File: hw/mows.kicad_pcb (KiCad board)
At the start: 2 copper layers, 47 x 50.8 mm, 18 parts, among them J1 ICSP, J2 STX882, J3 DHT22, J4 WSPD, J5 WDIR, J6 RAIN, U1 MCP1700, U2 ATTINY85-20PU

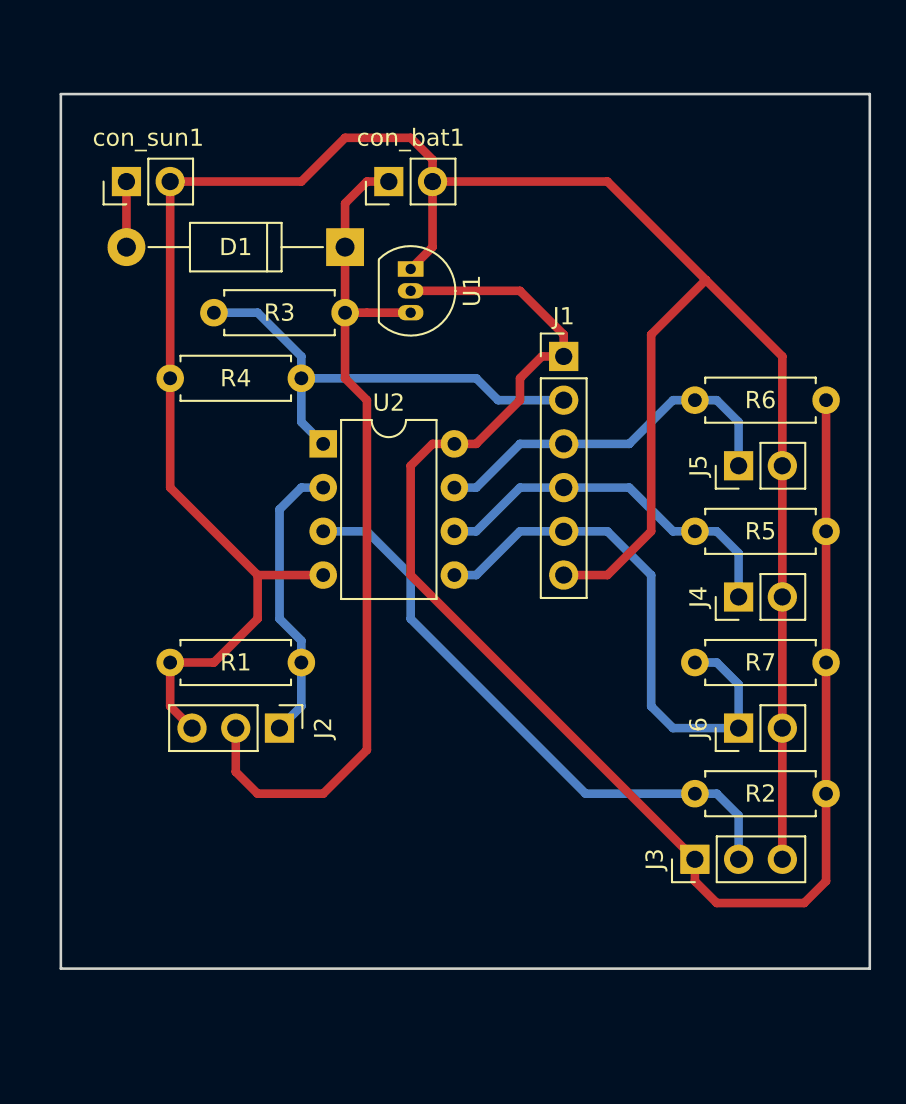
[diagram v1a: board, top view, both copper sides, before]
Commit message: Nova placa
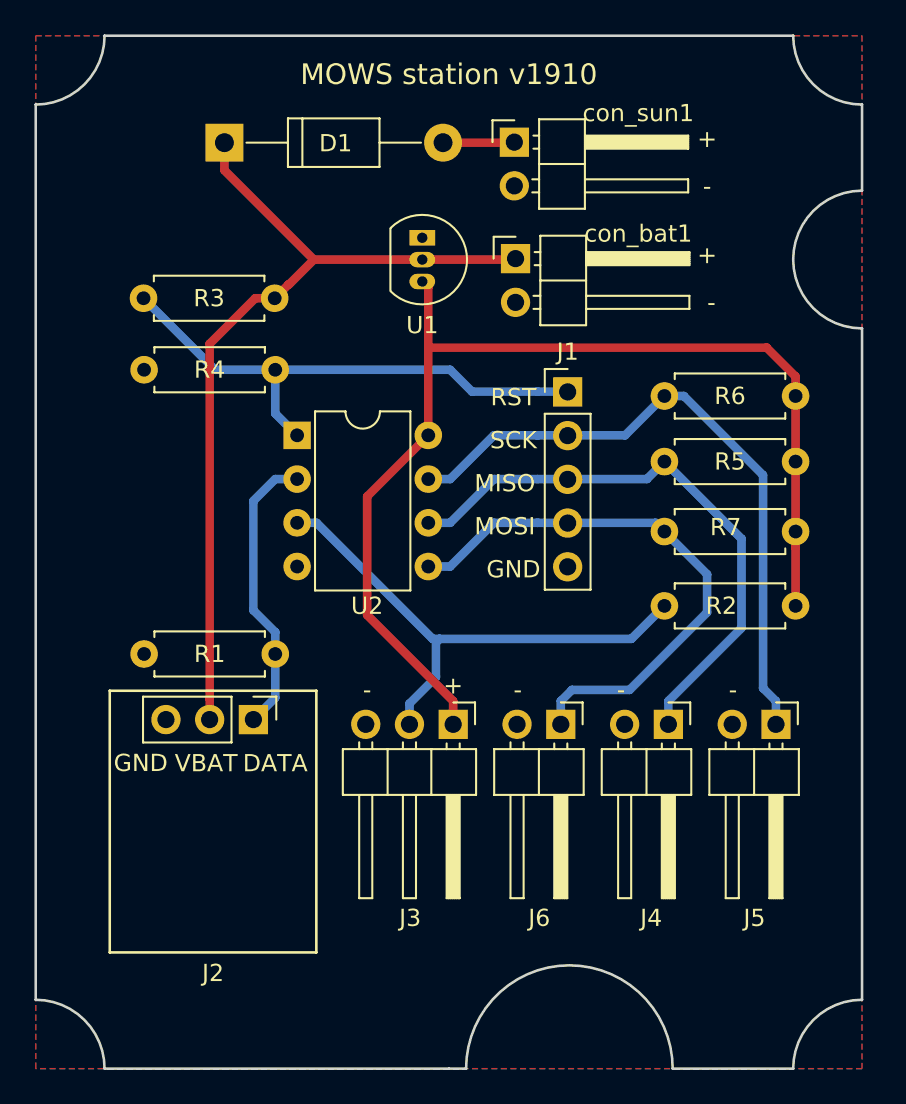
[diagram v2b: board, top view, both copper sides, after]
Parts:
- D1: value shottky -> D_Schottky
- J1: value ICSP -> Conn_01x05; footprint Pin_Headers:Pin_Header_Straight_1x06_Pitch2.54mm -> Connector_PinHeader_2.54mm:PinHeader_1x05_P2.54mm_Vertical
- J3: footprint Pin_Headers:Pin_Header_Straight_1x03_Pitch2.54mm -> Connector_PinHeader_2.54mm:PinHeader_1x03_P2.54mm_Horizontal
- J4, J5, J6, con_bat1, con_sun1: footprint Pin_Headers:Pin_Header_Straight_1x02_Pitch2.54mm -> Connector_PinHeader_2.54mm:PinHeader_1x02_P2.54mm_Horizontal
- U1: value MCP1700 -> MCP1700-3302E_TO92
- moved con_sun1 22.6 mm to (150.8, 75.2), turned to 0 degrees
- moved J3 16.1 mm to (147.2, 109.0), turned to 270 degrees
- moved J5 15.2 mm to (166.0, 109.0), turned to 270 degrees
- moved R2 11.1 mm to (167.1, 102.1)
- moved J6 10.3 mm to (153.5, 109.0), turned to 270 degrees
- moved D1 9.27 mm to (134.0, 75.2), turned to 0 degrees
- moved con_bat1 8.62 mm to (150.9, 81.9), turned to 0 degrees
- moved J4 8.45 mm to (159.8, 109.0), turned to 270 degrees
- moved R7 7.81 mm to (167.1, 97.8)
- moved R5 4.42 mm to (167.1, 93.7)
- moved R3 4.17 mm to (136.9, 84.2)
- moved J1 2.07 mm to (153.9, 89.7)
- moved U1 1.93 mm to (145.5, 80.7)
- moved R6 1.79 mm to (167.1, 89.9)
- moved R4 1.60 mm to (136.9, 88.4)
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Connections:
- net /SUN renamed Net-(D1-Pad2)
- J1 pad 1: +3V3 -> /RST
- J1 pad 2: /RST -> /SCK
- J1 pad 3: /SCK -> /MISO
- J1 pad 4: /MISO -> /MOSI
- J1 pad 5: /MOSI -> GND
- U1 pad 2: +3V3 -> +BATT
- U1 pad 3: +BATT -> +3V3
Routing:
- net GND: track 141.3 -> 0.00 mm
- net +3V3: track 91.1 -> 65.7 mm
- net /SCK: track 21.7 -> 38.1 mm
- net /MISO: track 21.7 -> 34.1 mm
- net /DHT22: track 35.0 -> 30.6 mm
- net /RST: track 27.5 -> 31.5 mm
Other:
- board size 47 x 50.8 mm -> 48 x 60 mm
- board text added: "+"
- board text added: "-"
- board text added: "DATA"
- board text added: "GND"
- board text added: "MISO"
- board text added: "MOSI"
- board text added: "MOWS station v1910"
- board text added: "RST"
- board text added: "SCK"
- board text added: "VBAT"
